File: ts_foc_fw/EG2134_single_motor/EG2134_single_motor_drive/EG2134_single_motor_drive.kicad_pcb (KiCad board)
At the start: 4 copper layers, 61.3 x 22.9 mm, 61 parts, among them CN1 XT30PW-M, CN2 WAFER-GH1.25-10PWB, Q1 RU3089M-C, Q2 RU3089M-C, Q3 RU3089M-C, Q4 RU3089M-C, Q5 RU3089M-C, Q6 RU3089M-C, U1 EG2134_N, U2 SY8205FCC, U3 TP181A1-CR, U4 TP181A1-CR, U5 MR30PW-M30.G.Y

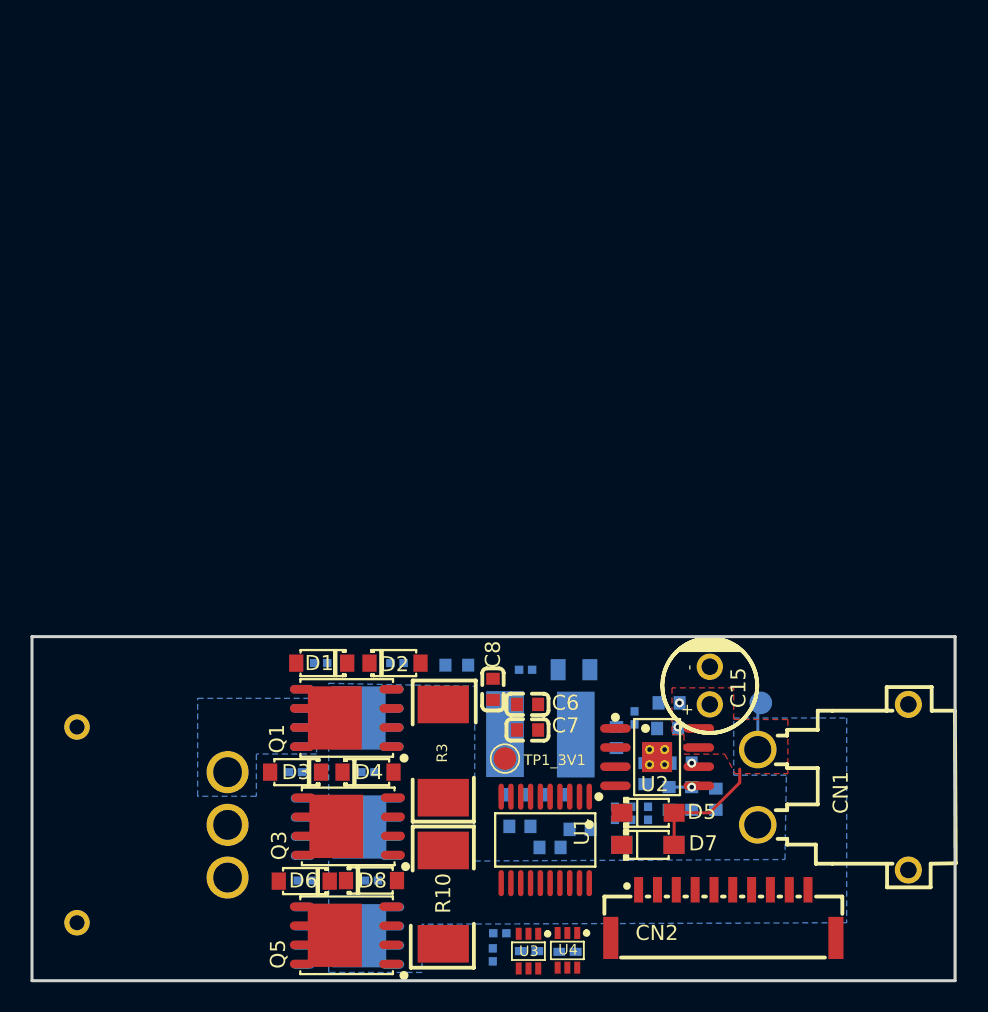
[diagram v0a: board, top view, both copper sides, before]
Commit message: 第一版走线完成,准备打板子验证
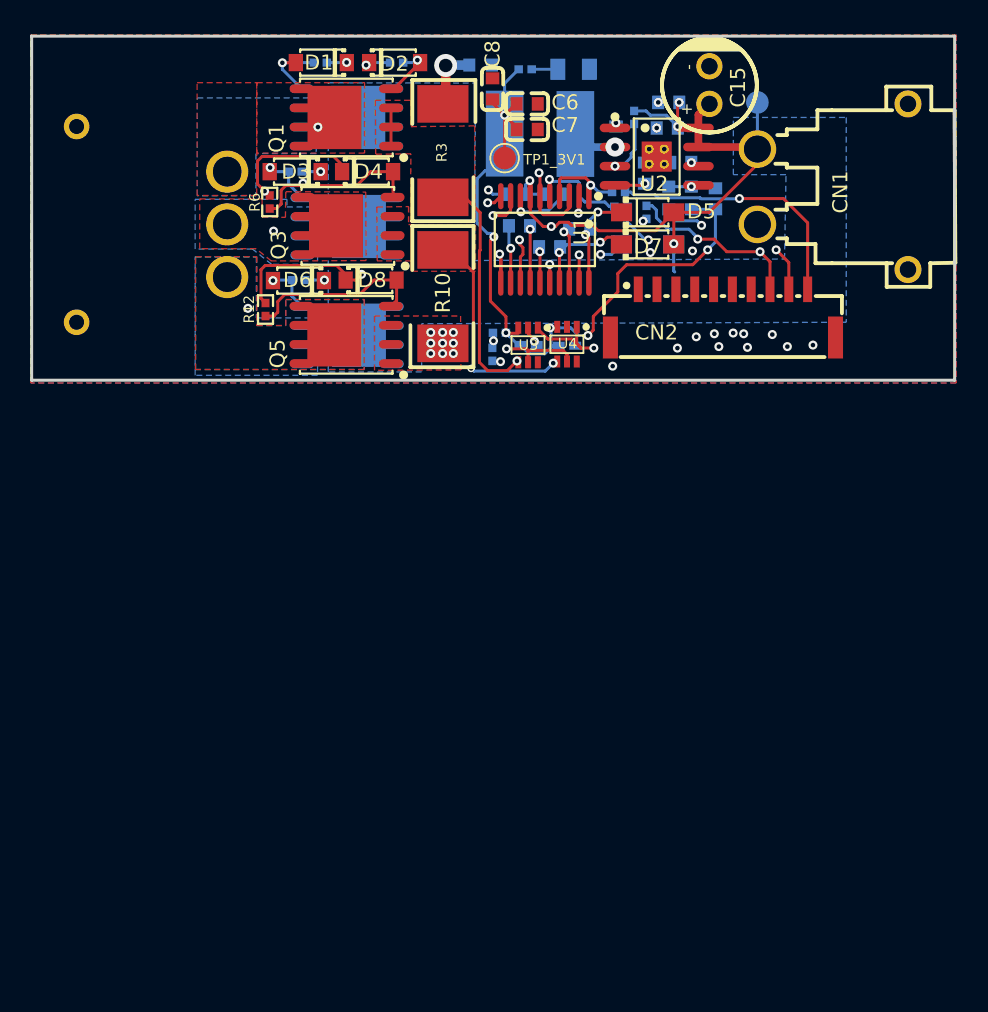
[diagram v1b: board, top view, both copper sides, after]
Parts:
- R12, R6: moved to F.Cu
- moved R7 41.3 mm to (51.0, 22.4), turned to 180 degrees
- moved R8 40.3 mm to (51.1, 23.3), turned to 180 degrees
- moved C16 40.3 mm to (45.0, 32.5)
- moved C17 40.3 mm to (47.5, 32.6)
- moved U3 40.3 mm to (44.9, 32.5)
- moved U4 40.3 mm to (47.5, 32.5)
- moved R9 40.0 mm to (52.8, 23.7)
- moved R4 39.9 mm to (41.8, 13.9)
- moved D6 39.9 mm to (29.7, 28.3)
- moved R11 39.9 mm to (29.7, 28.2)
- moved TP2_VCC1 39.9 mm to (60.2, 16.4)
- moved C4 39.9 mm to (46.4, 26.0)
- moved U1 39.9 mm to (46.1, 25.5)
- moved U5 39.9 mm to (20.0, 24.5)
- moved C1 39.9 mm to (46.7, 22.5)
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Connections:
- U2 pad : (no net) -> GND
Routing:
- net +3V3: track 0.00 -> 53.5 mm, vias 0 -> 6
- net VCC: track 11.7 -> 44.1 mm, vias 2 -> 5
- net HO1: track 0.00 -> 26.8 mm, vias 0 -> 2
- net LO2: track 0.00 -> 25.7 mm, vias 0 -> 2
- net V: track 0.00 -> 24.8 mm, vias 0 -> 2
- net VS3: track 0.00 -> 24.2 mm, vias 0 -> 2
- net GND: track 0.00 -> 24.1 mm, vias 0 -> 20
- net U: track 0.00 -> 23.1 mm, vias 0 -> 2
- net HO2: track 0.00 -> 23.0 mm, vias 0 -> 2
- net LO3: track 0.00 -> 22.5 mm, vias 0 -> 2
- net LO1: track 0.00 -> 22.5 mm, vias 0 -> 2
- net IS1: track 0.00 -> 20.2 mm, vias 0 -> 1
- net HO3: track 0.00 -> 19.7 mm, vias 0 -> 2
- net IN_1: track 0.00 -> 17.4 mm, vias 0 -> 1
- net VREF: track 0.00 -> 16.8 mm, vias 0 -> 2
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- added copper zone on B.Cu, net GND
- added copper zone on F.Cu, net GND
- added copper zone on F.Cu, net IS1
- added copper zone on F.Cu, net IS2
- added copper zone on F.Cu, net PGND
- added copper zone on In1.Cu, net PGND
- added copper zone on F.Cu, net U
- added copper zone on B.Cu, net V
- added copper zone on F.Cu, net V
- added copper zone on B.Cu, net VS3
- added copper zone on F.Cu, net VS3
- removed copper zone on F.Cu, net VCC
